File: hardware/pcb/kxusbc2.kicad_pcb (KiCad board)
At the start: 4 copper layers, 69 x 19 mm, 98 parts, among them J1 Conn_01x03, J2 UPDI, J3 Conn_01x03, J4 Conn_01x03, J5 GT-USB-7055AB, J6 Serial, J7 Conn_01x01, J8 Conn_01x01, Q1 CSD17581Q3A, Q2 CSD17581Q3A, Q3 CSD17581Q3A, Q4 CSD17581Q3A, Q5 CSD25402Q3A, SW1 SW_Push, U1 BQ25792RQMR, U2 ATtiny3226-M, U3 TLV9301xDCK, U4 RT9058-33GV, U5 LP5815DRLR, U7 FUSB302BMPX, Y1 32.768 kHz

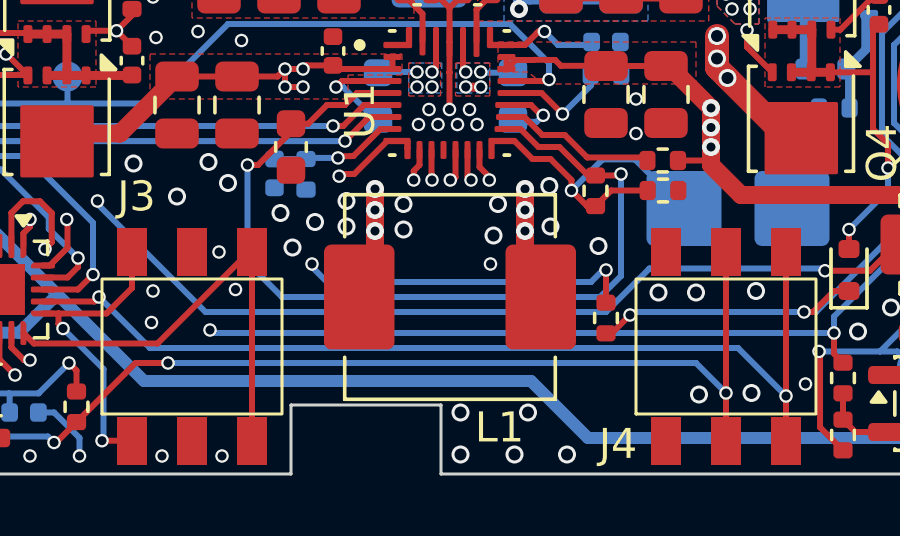
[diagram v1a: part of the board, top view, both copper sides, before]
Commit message: Move inductor slightly away from bottom edge
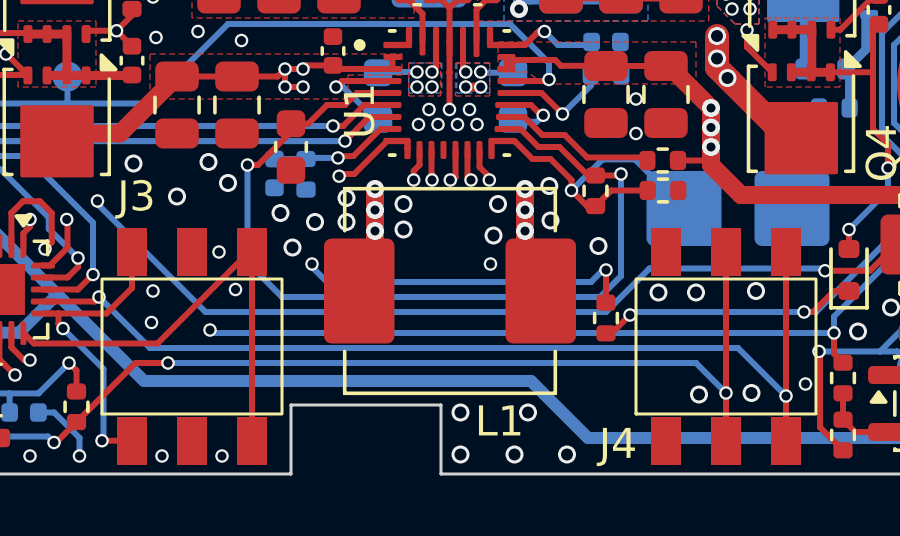
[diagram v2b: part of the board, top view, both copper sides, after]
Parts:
- moved L1 0.20 mm to (137.1, 118.7)
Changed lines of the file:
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@@
 	(footprint "Inductor_SMD:L_APV_APH0630"
 		(layer "F.Cu")
-		(at 137.1 118.9 180)
+		(at 137.1 118.7 180)
 		(descr "Inductor, APV, APH0630, 6.8x6.6x2.8mm, (http://en.apvind.com/public/upload/20240408/996aafa961154ed753e4983e7eb80fa7.pdf), generated with kicad-footprint-generator gen_inductor.py")
 		(tags "molded power shielded")
@@
 	)
 	(via
-		(at 140.45 116.55)
+		(at 140.45 116.35)
 		(size 0.6)
 		(drill 0.4)
@@
 	)
 	(via
-		(at 133.65 115.7)
+		(at 133.65 115.6)
 		(size 0.6)
 		(drill 0.4)
@@
 	)
 	(via
-		(at 133.65 116.55)
+		(at 133.65 116.4)
 		(size 0.6)
 		(drill 0.4)
@@
 	)
 	(segment
-		(start 134.05 118.9)
-		(end 134.6 118.35)
+		(start 134.075 118.7)
+		(end 134.6 118.175)
 		(width 0.6)
 		(layer "F.Cu")
@@
 	)
 	(segment
-		(start 134.6 118.35)
+		(start 134.6 118.175)
 		(end 134.6 115.299997)
 		(width 0.6)
@@
 	)
 	(segment
+		(start 139.6 118.175)
+		(end 139.6 115.3)
+		(width 0.6)
+		(layer "F.Cu")
+		(net 29)
+	)
+	(segment
+		(start 140.125 118.7)
+		(end 139.6 118.175)
+		(width 0.6)
+		(layer "F.Cu")
+		(net 29)
+	)
+	(segment
 		(start 137.53375 111.25)
 		(end 137.53375 110.4)
@@
 		(layer "F.Cu")
 		(net 29)
-	)
-	(segment
-		(start 139.6 118.9)
-		(end 139.6 115.3)
-		(width 0.6)
-		(layer "F.Cu")
-		(net 29)
